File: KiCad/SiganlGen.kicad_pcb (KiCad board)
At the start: 2 copper layers, 96.5 x 67.3 mm, 90 parts, among them J1 Barrel_Jack_MountingPin, J2 Conn_Coaxial, J3 LCD_Conn, J4 Enc_Conn, J6 Btn&Led, J7 PWR, J9 Btn_Matrix, Q1 BD135, Q2 BD136, U1 RaspberryPi_Pico, U2 MC34063AP, U3 LM7805_TO220, U4 LM337_TO220, U6 LM318H, U7 LM317_TO-220

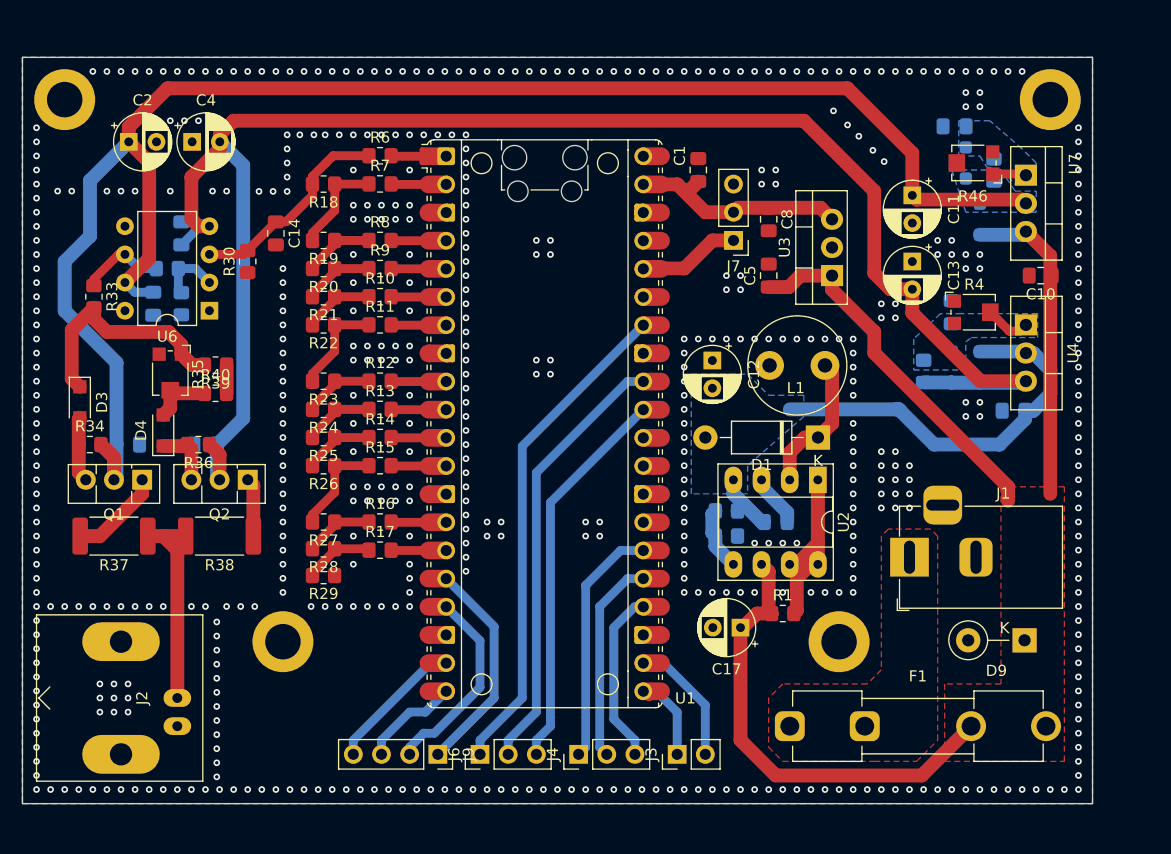
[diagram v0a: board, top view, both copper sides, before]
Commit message: Final PCB version (probably)
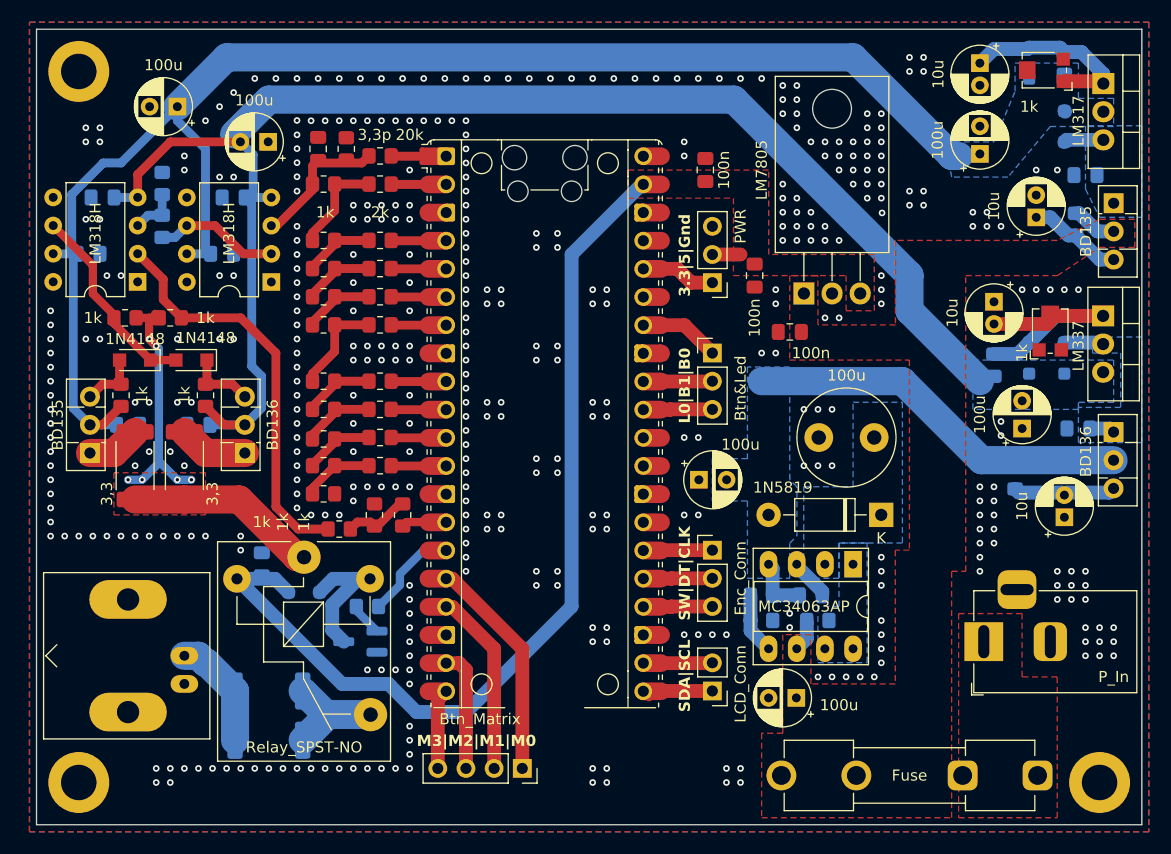
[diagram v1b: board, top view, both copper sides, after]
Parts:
- removed D1: 1N5819, Diode_THT:D_DO-41_SOD81_P10.16mm_Horizontal
- removed J9: Btn_Matrix, Connector_PinSocket_2.54mm:PinSocket_1x04_P2.54mm_Vertical
- removed R45: 100, Resistor_SMD:R_0805_2012Metric_Pad1.20x1.40mm_HandSolder
- removed R46: 1k, Potentiometer_SMD:Potentiometer_Bourns_TC33X_Vertical
- removed the REF** at (114.3, 38.1)
- added C20: 100n, Capacitor_SMD:C_0805_2012Metric_Pad1.18x1.45mm_HandSolder, B.Cu at (116.4, 52.0)
- added C21: 100n, Capacitor_SMD:C_0805_2012Metric_Pad1.18x1.45mm_HandSolder, B.Cu at (117.7, 46.9)
- added C22: 100u, Capacitor_THT:CP_Radial_D5.0mm_P2.50mm, F.Cu at (124.5, 38.7)
- added C23: 100u, Capacitor_THT:CP_Radial_D5.0mm_P2.50mm, F.Cu at (132.7, 41.9)
- added C24: 100n, Capacitor_SMD:C_0805_2012Metric_Pad1.18x1.45mm_HandSolder, B.Cu at (132.1, 80.0)
- added D5: 1N4007, Diode_SMD:D_SOD-123F, B.Cu at (201.3, 34.8)
- added J5: Enc_Conn, Connector_PinHeader_2.54mm:PinHeader_1x03_P2.54mm_Vertical, F.Cu at (172.7, 78.7)
- added K1: Relay_SPST-NO, Relay_THT:Relay_SPST_SANYOU_SRD_Series_Form_B, F.Cu at (135.9, 79.4)
- added Q4: BD135, Package_TO_SOT_THT:TO-126-3_Vertical, F.Cu at (116.6, 70.0)
- added Q5: BD136, Package_TO_SOT_THT:TO-126-3_Vertical, F.Cu at (130.6, 70.0)
- added Q6: BC817, Package_TO_SOT_SMD:SOT-23_Handsoldering, B.Cu at (141.0, 87.0)
- added R41: 1k, Resistor_SMD:R_0805_2012Metric_Pad1.20x1.40mm_HandSolder, F.Cu at (119.7, 57.8)
- added R42: 3,3, Resistor_SMD:R_2512_6332Metric_Pad1.40x3.35mm_HandSolder, F.Cu at (120.7, 71.1)
- added R43: 3,3, Resistor_SMD:R_2512_6332Metric_Pad1.40x3.35mm_HandSolder, F.Cu at (125.1, 71.1)
- added R44: 1k, Resistor_SMD:R_0805_2012Metric_Pad1.20x1.40mm_HandSolder, B.Cu at (123.1, 45.7)
- added U5: LM337, Package_TO_SOT_THT:TO-220-3_Vertical, F.Cu at (208.0, 57.6)
- C10, R1: moved to B.Cu
- C11, C12: value 100u -> 10u; footprint Capacitor_THT:CP_Radial_D5.0mm_P2.50mm -> Capacitor_THT:CP_Radial_D5.0mm_P2.00mm
- C14: value 3,3p -> 100u; footprint Capacitor_SMD:C_0805_2012Metric_Pad1.18x1.45mm_HandSolder -> Capacitor_THT:CP_Radial_D5.0mm_P2.50mm
- C15: value 100n -> 3,3p; moved to F.Cu
- C17: value 100u -> 100n; footprint Capacitor_THT:CP_Radial_D5.0mm_P2.50mm -> Capacitor_SMD:C_0805_2012Metric_Pad1.18x1.45mm_HandSolder; moved to B.Cu
- C4: value 100u -> 100n; footprint Capacitor_THT:CP_Radial_D5.0mm_P2.50mm -> Capacitor_SMD:C_0805_2012Metric_Pad1.18x1.45mm_HandSolder
- C6: value 10u -> 100u; footprint Capacitor_SMD:C_0805_2012Metric_Pad1.18x1.45mm_HandSolder -> Capacitor_THT:CP_Radial_D5.0mm_P2.50mm; moved to F.Cu
- C7: value 100n -> 10u; footprint Capacitor_SMD:C_0805_2012Metric_Pad1.18x1.45mm_HandSolder -> Capacitor_THT:CP_Radial_D5.0mm_P2.00mm; moved to F.Cu
- C8: value 100n -> 10u; footprint Capacitor_SMD:C_0805_2012Metric_Pad1.18x1.45mm_HandSolder -> Capacitor_THT:CP_Radial_D5.0mm_P2.00mm
- C9: value 10u -> 100n
- D2: value 1N4007 -> 1N5819; footprint Diode_SMD:D_SOD-123F -> Diode_THT:D_DO-41_SOD81_P10.16mm_Horizontal; moved to F.Cu
- D3, D4: value 1N4148 -> 1N4007; footprint Diode_SMD:Nexperia_CFP3_SOD-123W -> Diode_SMD:D_SOD-123F; moved to B.Cu
- D8: value 1N4007 -> 1N4148; footprint Diode_SMD:D_SOD-123F -> Diode_SMD:Nexperia_CFP3_SOD-123W; moved to F.Cu
- D9: value 1N4148WT -> 1N4148; footprint Diode_THT:D_DO-41_SOD81_P5.08mm_Vertical_KathodeUp -> Diode_SMD:Nexperia_CFP3_SOD-123W
- J1: value Barrel_Jack_MountingPin -> P_In
- J3: value LCD_Conn -> Btn_Matrix; footprint Connector_PinHeader_2.54mm:PinHeader_1x02_P2.54mm_Vertical -> Connector_PinSocket_2.54mm:PinSocket_1x04_P2.54mm_Vertical
- J4: value Enc_Conn -> LCD_Conn; footprint Connector_PinHeader_2.54mm:PinHeader_1x03_P2.54mm_Vertical -> Connector_PinHeader_2.54mm:PinHeader_1x02_P2.54mm_Vertical
- R18, R19: value 1k -> 2k
- R2: value 1,5k -> 2k
- R3: value 14k -> 18k
- R30: value 20k -> 1k
- R31: value 680 -> 1k; moved to F.Cu
- R32: value 680 -> 20k; moved to F.Cu
- R33: value 27 -> 100; moved to B.Cu
- R35: value 1k -> 100; footprint Potentiometer_SMD:Potentiometer_Bourns_TC33X_Vertical -> Resistor_SMD:R_2512_6332Metric_Pad1.40x3.35mm_HandSolder; moved to B.Cu
- R36: value 1k -> 100; footprint Resistor_SMD:R_0805_2012Metric_Pad1.20x1.40mm_HandSolder -> Resistor_SMD:R_2512_6332Metric_Pad1.40x3.35mm_HandSolder; moved to B.Cu
- R37: value 3,3 -> 1k; footprint Resistor_SMD:R_2512_6332Metric_Pad1.40x3.35mm_HandSolder -> Resistor_SMD:R_0805_2012Metric_Pad1.20x1.40mm_HandSolder; moved to B.Cu
- R38: value 3,3 -> 1k; footprint Resistor_SMD:R_2512_6332Metric_Pad1.40x3.35mm_HandSolder -> Resistor_SMD:R_0805_2012Metric_Pad1.20x1.40mm_HandSolder
- R39, R40, R5: value 100 -> 1k
- R4: footprint Potentiometer_SMD:Potentiometer_Bourns_TC33X_Vertical -> Resistor_SMD:R_0805_2012Metric_Pad1.20x1.40mm_HandSolder; moved to B.Cu
- R6, R7: value 2k -> 1k; footprint Resistor_SMD:R_0805_2012Metric_Pad1.20x1.40mm_HandSolder -> Potentiometer_SMD:Potentiometer_Bourns_TC33X_Vertical
- R8, R9: value 2k -> 100; moved to B.Cu
- U3: value LM7805_TO220 -> LM7805; footprint Package_TO_SOT_THT:TO-220-3_Vertical -> Package_TO_SOT_THT:TO-220-3_Horizontal_TabDown
- U4: value LM337_TO220 -> LM317
- U7: value LM317_TO-220 -> LM318H; footprint Package_TO_SOT_THT:TO-220-3_Vertical -> Package_DIP:DIP-8_W7.62mm
- moved REF** 107.1 mm to (115.6, 99.7)
- moved Q1 91.1 mm to (208.9, 47.4), turned to -90 degrees
- moved D3 88.9 mm to (204.5, 61.4), turned to 90 degrees
- moved D4 85.8 mm to (204.5, 40.5)
- moved REF** 85.7 mm to (115.6, 35.6)
- moved U7 80.7 mm to (120.9, 54.5), turned to 180 degrees
- moved D9 79.3 mm to (125.7, 61.6)
- moved C2 78.4 mm to (180.3, 92.1), turned to 180 degrees
- moved Q2 78.2 mm to (208.9, 68.1), turned to -90 degrees
- moved REF** 74.7 mm to (207.6, 99.7)
- moved D8 73.7 mm to (120.7, 61.6), turned to 180 degrees
- moved D7 71.2 mm to (135.9, 82.5), turned to 0 degrees
- moved C14 69.6 mm to (200.7, 67.8), turned to 90 degrees
- moved R8 63.8 mm to (204.5, 34.8), turned to -90 degrees
- moved R7 61.9 mm to (203.2, 58.9), turned to 90 degrees
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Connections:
- C10 pad 1: +12V -> GND
- C10 pad 2: GND -> Net-(D3-A)
- C11 pad 1: +10V -> Net-(D5-A)
- C12 pad 2: -12V -> Net-(D6-K)
- C13 pad 1: GND -> +10V
- C13 pad 2: -10V -> GND
- C14 pad 1: /Output Stage/DAC_OUT -> GND
- C14 pad 2: GND -> -10V
- C15 pad 1: +10V -> /Output Stage/DAC_OUT
- C16 pad 1: GND -> +10V
- C16 pad 2: -10V -> GND
- C17 pad 1: +12V -> GND
- C17 pad 2: GND -> -10V
- C2 pad 1: +10V -> +12V
- C4 pad 1: GND -> +12V
- C4 pad 2: -10V -> GND
- C5 pad 1: +12V -> +5V
- C6 pad 1: Net-(D7-A) -> GND
- C6 pad 2: GND -> -12V
- C7 pad 1: GND -> Net-(Q1-B)
- C7 pad 2: -12V -> GND
- C8 pad 1: +5V -> GND
- C8 pad 2: GND -> Net-(Q2-B)
- C9 pad 1: GND -> Net-(D4-K)
- C9 pad 2: Net-(D8-K) -> GND
- D2 pad 1: -10V -> Net-(D2-K)
- D3 pad 1: Net-(D3-K) -> -10V
- D4 pad 2: Net-(D4-A) -> +10V
- D6 pad 1: +12V -> Net-(D6-K)
- D6 pad 2: +10V -> -10V
- D7 pad 1: +10V -> +5V
- D8 pad 2: -10V -> Net-(D8-A)
- D9 pad 1: +12V -> Net-(D9-K)
- D9 pad 2: GND -> Net-(D8-K)
- J3 pad 1: /LCD.SDA -> /MUX0
- J3 pad 2: /LCD.SCL -> /MUX1
- J4 pad 1: /ENC.CLK -> /LCD.SDA
- J4 pad 2: /ENC.DT -> /LCD.SCL
- L1 pad 1: Net-(D1-K) -> Net-(D2-K)
- Q1 pad 1: Net-(Q1-E) -> Net-(D4-K)
- Q1 pad 2: +10V -> +12V
- Q1 pad 3: Net-(D3-A) -> Net-(Q1-B)
- Q2 pad 1: Net-(Q2-E) -> Net-(D3-A)
- Q2 pad 2: -10V -> -12V
- Q2 pad 3: Net-(D4-K) -> Net-(Q2-B)
- R10 pad 1: Net-(R10-Pad1) -> /Output Stage/DAC_OUT
- R10 pad 2: /DAC4 -> /DAC0
- R11 pad 2: /DAC5 -> /DAC1
- R12 pad 2: /DAC6 -> /DAC2
- R13 pad 2: /DAC7 -> /DAC3
- R14 pad 2: /DAC8 -> /DAC4
- R15 pad 2: /DAC9 -> /DAC5
- R16 pad 2: /DAC10 -> /DAC6
- R17 pad 2: /DAC11 -> /DAC7
- R18 pad 2: /Output Stage/DAC_OUT -> /DAC8
- R19 pad 2: Net-(R18-Pad1) -> /DAC9
- R20 pad 1: Net-(R20-Pad1) -> Net-(R11-Pad1)
- R20 pad 2: Net-(R19-Pad1) -> /Output Stage/DAC_OUT
- R21 pad 1: Net-(R10-Pad1) -> Net-(R12-Pad1)
- R21 pad 2: Net-(R20-Pad1) -> Net-(R11-Pad1)
- R22 pad 1: Net-(R11-Pad1) -> Net-(R13-Pad1)
- R22 pad 2: Net-(R10-Pad1) -> Net-(R12-Pad1)
- R23 pad 1: Net-(R12-Pad1) -> Net-(R14-Pad1)
- R23 pad 2: Net-(R11-Pad1) -> Net-(R13-Pad1)
- R24 pad 1: Net-(R13-Pad1) -> Net-(R15-Pad1)
- R24 pad 2: Net-(R12-Pad1) -> Net-(R14-Pad1)
- R25 pad 1: Net-(R14-Pad1) -> Net-(R16-Pad1)
- R25 pad 2: Net-(R13-Pad1) -> Net-(R15-Pad1)
- R26 pad 1: Net-(R15-Pad1) -> Net-(R17-Pad1)
- R26 pad 2: Net-(R14-Pad1) -> Net-(R16-Pad1)
- R27 pad 1: Net-(R16-Pad1) -> Net-(R18-Pad1)
- R27 pad 2: Net-(R15-Pad1) -> Net-(R17-Pad1)
- R28 pad 1: Net-(R17-Pad1) -> Net-(R19-Pad1)
- R28 pad 2: Net-(R16-Pad1) -> Net-(R18-Pad1)
- R29 pad 2: Net-(R17-Pad1) -> Net-(R19-Pad1)
- R30 pad 1: GND -> Net-(R30-Pad1)
- R30 pad 2: /Output Stage/DAC_OUT -> /Output Stage/3.3Sig
- R31 pad 2: Net-(U6--) -> Net-(R30-Pad1)
- R32 pad 1: Net-(U6--) -> GND
- R32 pad 2: Net-(R32-Pad2) -> /Output Stage/DAC_OUT
- R33 pad 1: Net-(R32-Pad2) -> /Output Stage/OUT_EN
- R33 pad 2: Net-(D3-K) -> Net-(Q6-B)
- R34 pad 1: Net-(D3-A) -> Net-(U7--)
- R34 pad 2: +10V -> Net-(R30-Pad1)
- R35 pad 1: Net-(D3-K) -> Net-(J2-In)
- R35 pad 2: Net-(D4-A) -> Net-(K1-Pad14)
- R36 pad 1: -10V -> Net-(J2-In)
- R36 pad 2: Net-(D4-K) -> Net-(K1-Pad14)
- R37 pad 1: Net-(J2-In) -> Net-(U7-+)
- R37 pad 2: Net-(Q1-E) -> Net-(U6--)
- R38 pad 1: Net-(Q2-E) -> Net-(U7--)
- R38 pad 2: Net-(J2-In) -> /Output Stage/AMP_OUT
- R39 pad 1: Net-(R39-Pad1) -> Net-(D8-A)
- R39 pad 2: Net-(D3-K) -> +10V
- R4 pad 1: GND -> +12V
- R4 pad 2: Net-(D8-K) -> Net-(Q1-B)
- R40 pad 1: Net-(D4-A) -> -10V
- R40 pad 2: Net-(R39-Pad1) -> Net-(D9-K)
- R5 pad 1: -10V -> -12V
- R5 pad 2: Net-(D8-K) -> Net-(Q2-B)
- R6 pad 1: /Output Stage/DAC_OUT -> Net-(D5-A)
- R6 pad 2: /DAC0 -> GND
- R7 pad 1: Net-(R18-Pad1) -> GND
- R7 pad 2: /DAC1 -> Net-(D6-K)
- R8 pad 1: Net-(R19-Pad1) -> Net-(D5-A)
- R8 pad 2: /DAC2 -> +10V
- R9 pad 1: Net-(R20-Pad1) -> -10V
- R9 pad 2: /DAC3 -> Net-(D6-K)
- U1 pad 14: /DAC10 -> /Output Stage/3.3Sig
- U1 pad 15: /DAC11 -> /Output Stage/OUT_EN
- U2 pad 2: Net-(D1-K) -> Net-(D2-K)
- U4 pad 1: Net-(D8-K) -> Net-(D5-A)
- U4 pad 2: -12V -> +10V
- U4 pad 3: -10V -> Net-(D4-K)
- U6 pad 6: Net-(R32-Pad2) -> Net-(U6--)
- U7 pad 1: Net-(D7-A) -> unconnected-(U7-BAL1-Pad1)
- U7 pad 2: +10V -> Net-(U7--)
- U7 pad 3: +12V -> Net-(U7-+)
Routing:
- net +12V: track 104.8 -> 7.04 mm
- net +5V: track 20.0 -> 87.6 mm
- net /Output Stage/AMP_OUT: track 0.00 -> 41.3 mm, vias 0 -> 6
- net /UI.OUT0: track 44.8 -> 7.27 mm
- net Net-(U7--): track 0.00 -> 36.7 mm
- net /UI.OUT1: track 39.5 -> 6.24 mm
- net /UI.IN0: track 35.1 -> 6.24 mm
- net Net-(D3-K): track 21.5 -> 0.00 mm
- net Net-(D6-K): track 0.00 -> 21.4 mm
- net Net-(U2-DC): track 20.7 -> 0.00 mm
- net Net-(D5-A): track 0.00 -> 17.3 mm
- net /ENC.CLK: track 22.0 -> 6.24 mm
- net -10V: track 147.6 -> 133.5 mm
- net Net-(K1-Pad14): track 0.00 -> 14.1 mm
- net Net-(D8-K): track 4.15 -> 18.1 mm
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- added copper zone on F.Cu, net +5V
- added copper zone on B.Cu, net -10V
- added copper zone on F.Cu, net /Output Stage/AMP_OUT
- added copper zone on B.Cu, net Net-(D2-K)
- added copper zone on B.Cu, net Net-(D3-A)
- added copper zone on B.Cu, net Net-(D4-K)
- added copper zone on B.Cu, net Net-(U2-DC)
- removed copper zone on B.Cu, net Net-(D7-A)
- removed copper zone on B.Cu, net Net-(D8-K)
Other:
- board size 96.5 x 67.3 mm -> 99.7 x 71.8 mm
- board text added: "3.3|5|Gnd"
- board text added: "L0|B1|B0"
- board text added: "M3|M2|M1|M0"
- board text added: "SDA|SCL"
- board text added: "SW|DT|CLK"
